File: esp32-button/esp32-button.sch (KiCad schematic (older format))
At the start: 12 parts, among them J3 Conn_01x02_Female, SW1 SW_Push, SW2 SW_Push, SW3 SW_Push, SW4 SW_Push, SW5 SW_Push, SW6 SW_Push, U1 XIAO-ESP32C

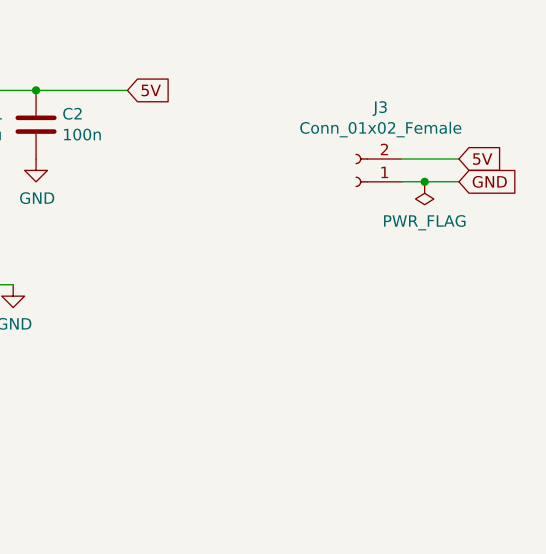
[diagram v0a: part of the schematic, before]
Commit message: sync
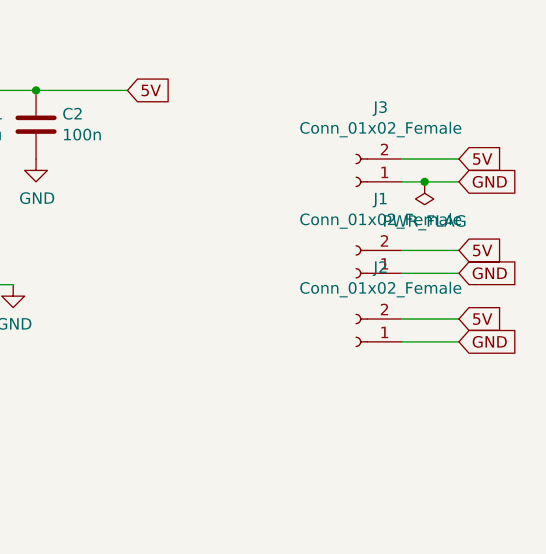
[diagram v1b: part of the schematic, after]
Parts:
- added J1, J2: Conn_01x02_Female, custom-footprints:solder-pad-2p, symbol Connector:Conn_01x02_Female
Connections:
- net 5V: now also J1.2 (Pin_2), J2.2 (Pin_2)
- net GND: now also J1.1 (Pin_1), J2.1 (Pin_1)
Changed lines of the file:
@@
 Wire Wire Line
 	4450 1800 4450 2050
+$Comp
+L Connector:Conn_01x02_Female J1
+U 1 1 6369FDD5
+P 6900 2000
+F 0 "J1" H 6792 1675 50  0000 C CNN
+F 1 "Conn_01x02_Female" H 6792 1766 50  0000 C CNN
+F 2 "custom-footprints:solder-pad-2p" H 6900 2000 50  0001 C CNN
+F 3 "~" H 6900 2000 50  0001 C CNN
+	1    6900 2000
+	-1   0    0    1
+$EndComp
+$Comp
+L Connector:Conn_01x02_Female J2
+U 1 1 636A0A9C
+P 6900 2300
+F 0 "J2" H 6792 1975 50  0000 C CNN
+F 1 "Conn_01x02_Female" H 6792 2066 50  0000 C CNN
+F 2 "custom-footprints:solder-pad-2p" H 6900 2300 50  0001 C CNN
+F 3 "~" H 6900 2300 50  0001 C CNN
+	1    6900 2300
+	-1   0    0    1
+$EndComp
+Text GLabel 7350 1900 2    50   Input ~ 0
+5V
+Text GLabel 7350 2000 2    50   Input ~ 0
+GND
+Text GLabel 7350 2200 2    50   Input ~ 0
+5V
+Text GLabel 7350 2300 2    50   Input ~ 0
+GND
+Wire Wire Line
+	7100 1900 7350 1900
+Wire Wire Line
+	7100 2000 7350 2000
+Wire Wire Line
+	7100 2200 7350 2200
+Wire Wire Line
+	7100 2300 7350 2300
 $EndSCHEMATC
